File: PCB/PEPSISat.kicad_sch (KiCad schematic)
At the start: 10 parts, among them J1 Conn_02x09_Counter_Clockwise, U1 STM32H747IITx, U2 RP2350A, U3 MT48LC16M16A2P, U4 BMP280, U5 LSM6DSOXTR

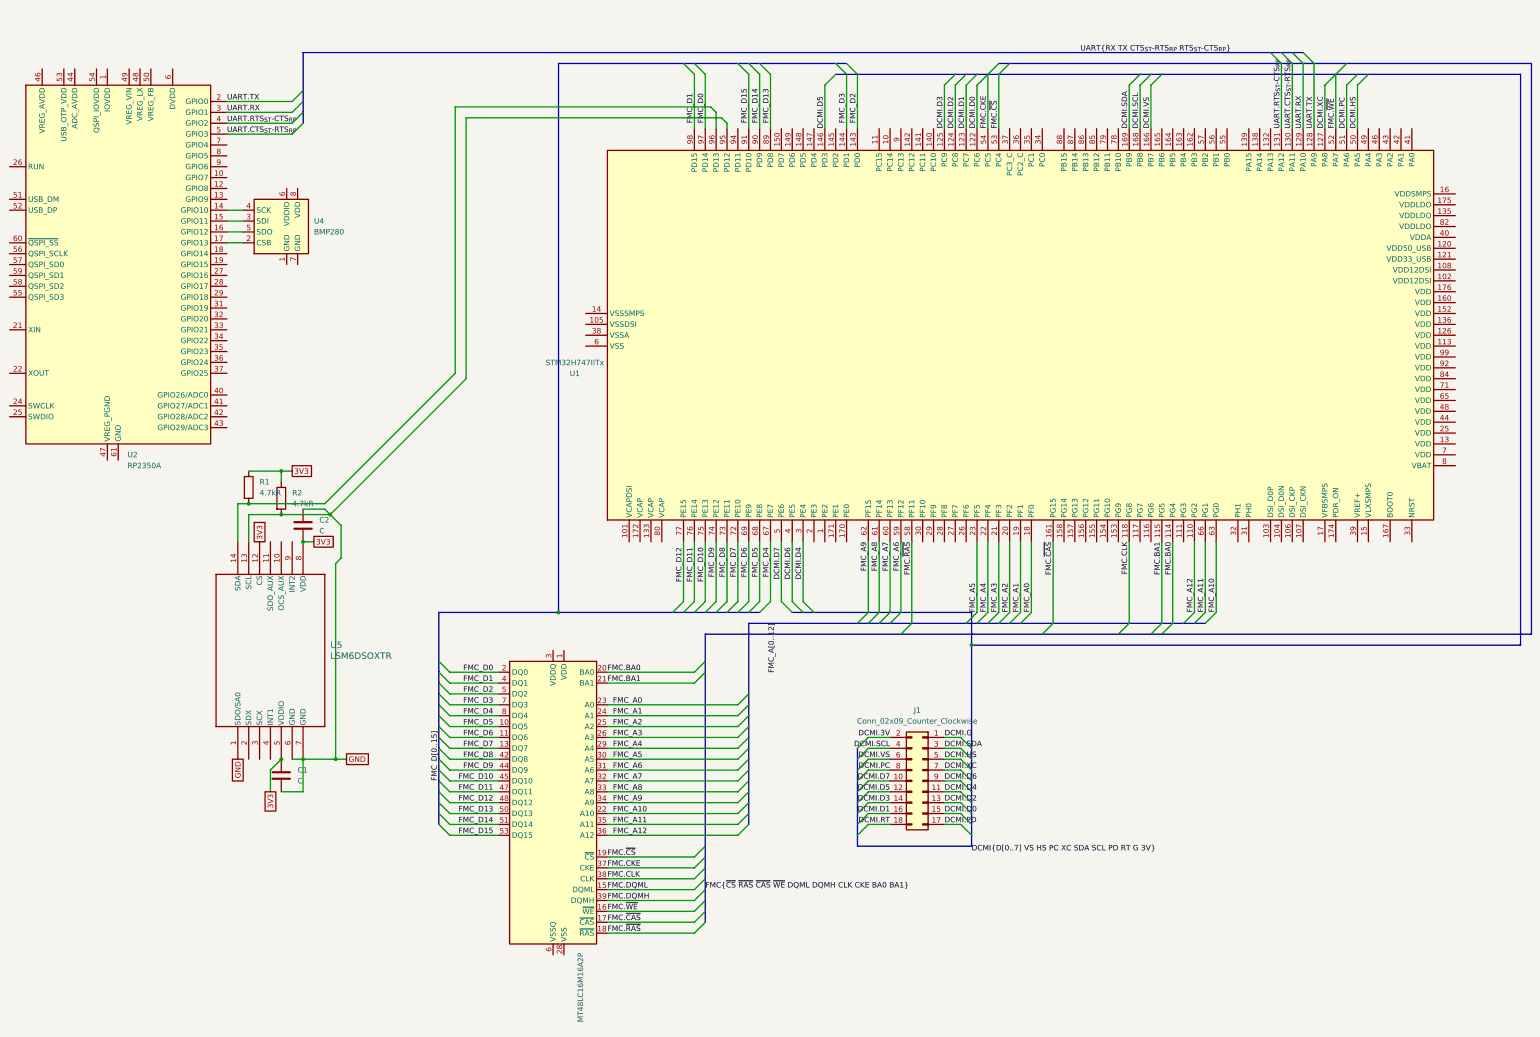
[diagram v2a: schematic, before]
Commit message: KiCad
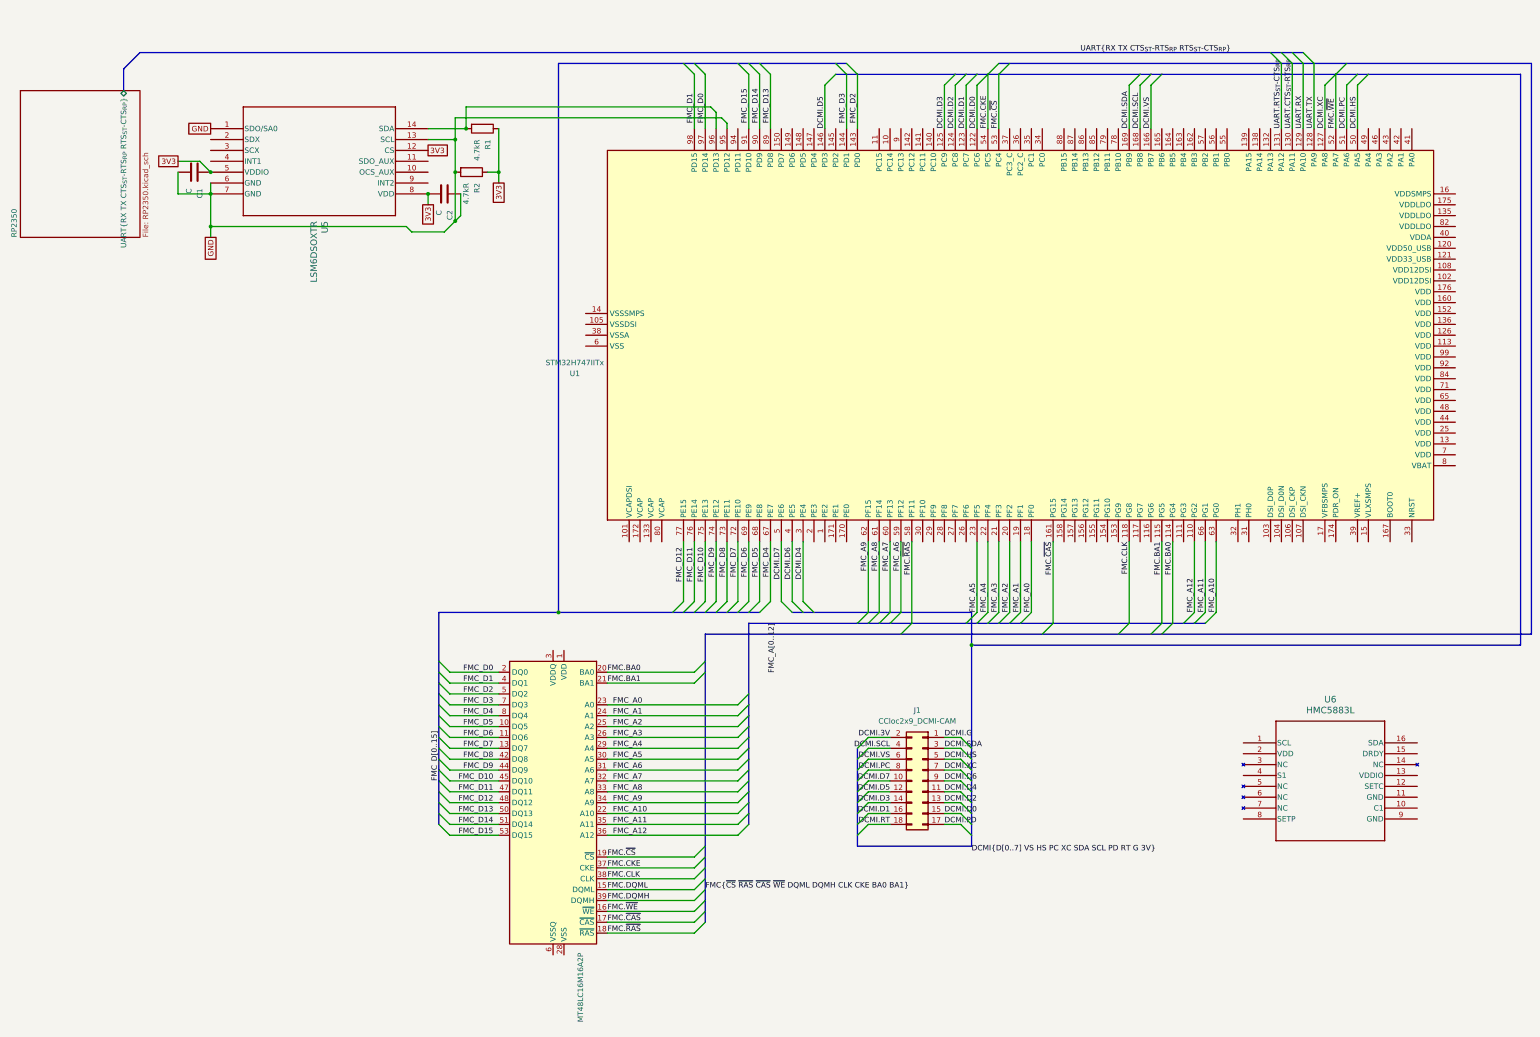
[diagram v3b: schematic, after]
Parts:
- removed U2: RP2350A, Package_DFN_QFN:QFN-60-1EP_7x7mm_P0.4mm_EP3.4x3.4mm, symbol MCU_RaspberryPi:RP2350A
- removed U4: BMP280, Package_LGA:Bosch_LGA-8_2x2.5mm_P0.65mm_ClockwisePinNumbering, symbol Sensor_Pressure:BMP280
- added U6: HMC5883L, LPCC16_HNW, symbol HMC5883L:HMC5883L
- J1: value Conn_02x09_Counter_Clockwise -> CCloc2x9_DCMI-CAM
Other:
- added sheet RP2350 (RP2350.kicad_sch)
- moved on the sheet: C1, C2, R1, R2, U5
